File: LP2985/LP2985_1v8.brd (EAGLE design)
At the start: 15.2 x 11.2 mm, 2 parts

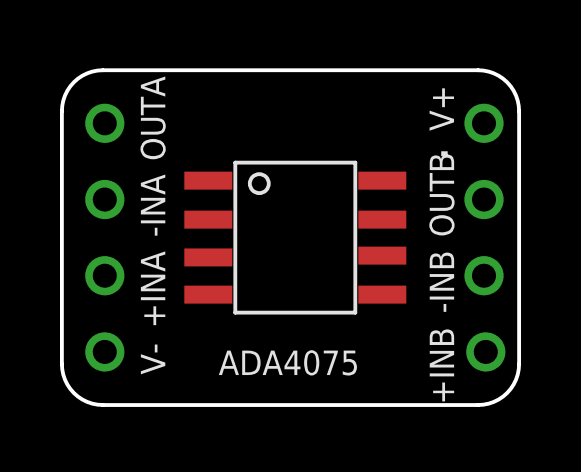
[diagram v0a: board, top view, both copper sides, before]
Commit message: Update new meme.
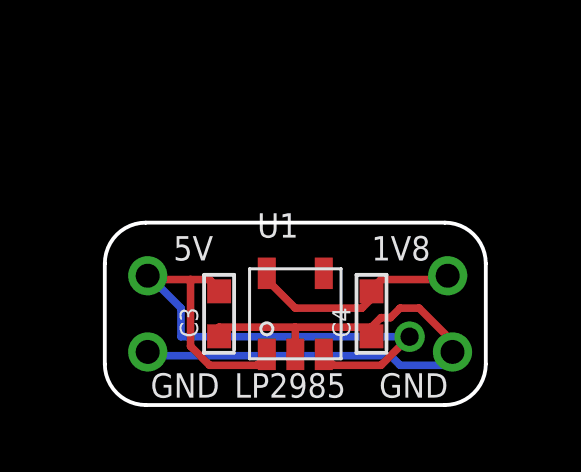
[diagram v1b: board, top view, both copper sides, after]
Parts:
- removed .: ADA4075, FaBo-Opamp:SOIC(NARROW)-8
- removed U$3: 8PIN, FaBo-Breakout:8PIN
- added C3, C4: 1uf, GClue-Capacitor:0603
- added U$2: 4PIN-REGULATOR, FaBo-Breakout:4PIN-REGULATOR
- added U1: (no value), FaBo-Supply:SOT_23_5
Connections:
- removed net 1: ..1, U$3.1
- removed net 2: ..2, U$3.2
- removed net 3: ..3, U$3.3
- removed net 4: ..4, U$3.4
- removed net 5: ..5, U$3.5
- removed net 6: ..6, U$3.6
- removed net 7: ..7, U$3.7
- removed net 8: ..8, U$3.8
- new net 5V: C3.2, U$2.V1, U1.1, U1.3
- new net GND: C3.1, C4.1, U$2.GND@1, U$2.GND@2, U1.2
- new net VCC: C4.2, U$2.V2, U1.5
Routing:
- net 5V: track 0.00 -> 21.4 mm, vias 0 -> 1
- net GND: track 0.00 -> 21.1 mm
- net VCC: track 0.00 -> 7.34 mm
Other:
- board size 15.2 x 11.2 mm -> 12.7 x 6.1 mm
- board text added: "1V8"
- board text added: "5V"
- board text added: "GND"
- board text added: "LP2985"
- board text removed: "+INA"
- board text removed: "+INB"
- board text removed: "-INA"
- board text removed: "-INB"
- board text removed: "ADA4075"
- board text removed: "OUTA"
- board text removed: "OUTB"
- board text removed: "V+"
- board text removed: "V-"
